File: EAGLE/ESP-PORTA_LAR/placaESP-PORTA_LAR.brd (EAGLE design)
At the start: 53.3 x 42.9 mm, 18 parts

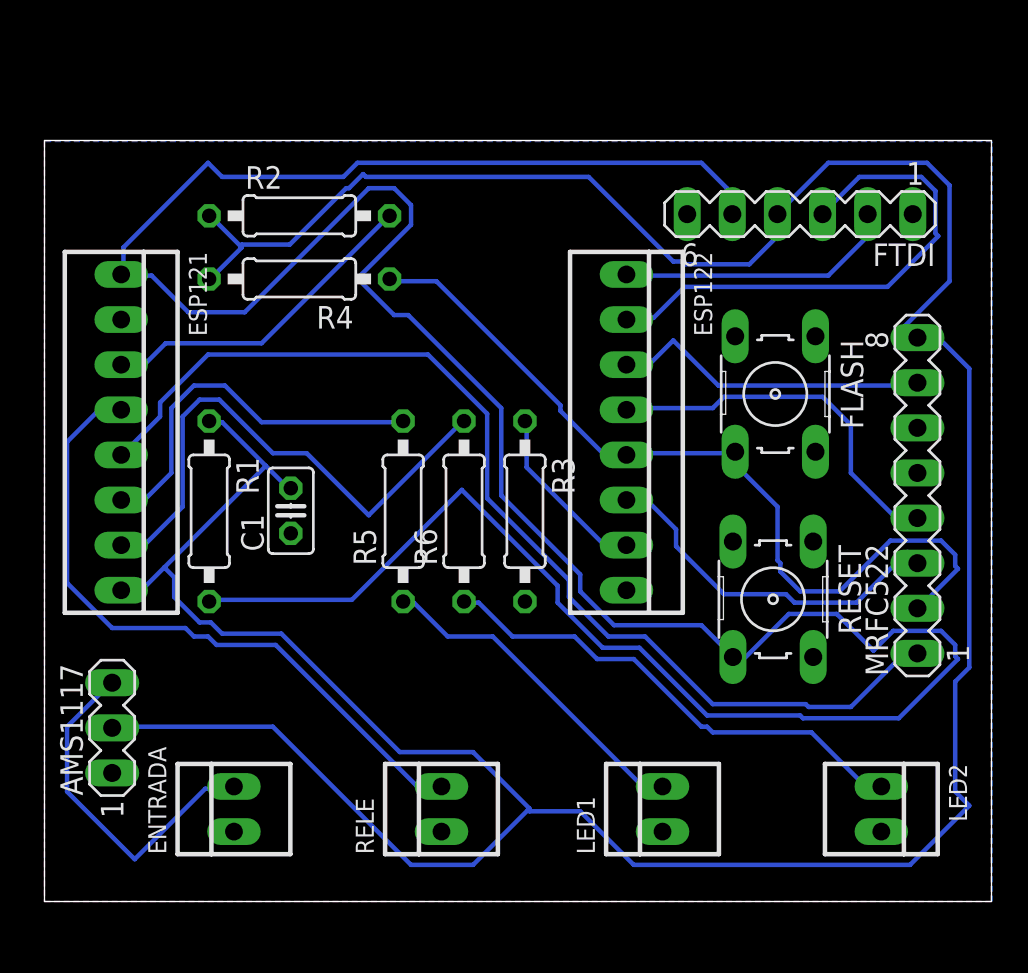
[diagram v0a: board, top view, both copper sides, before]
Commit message: Nova Placa
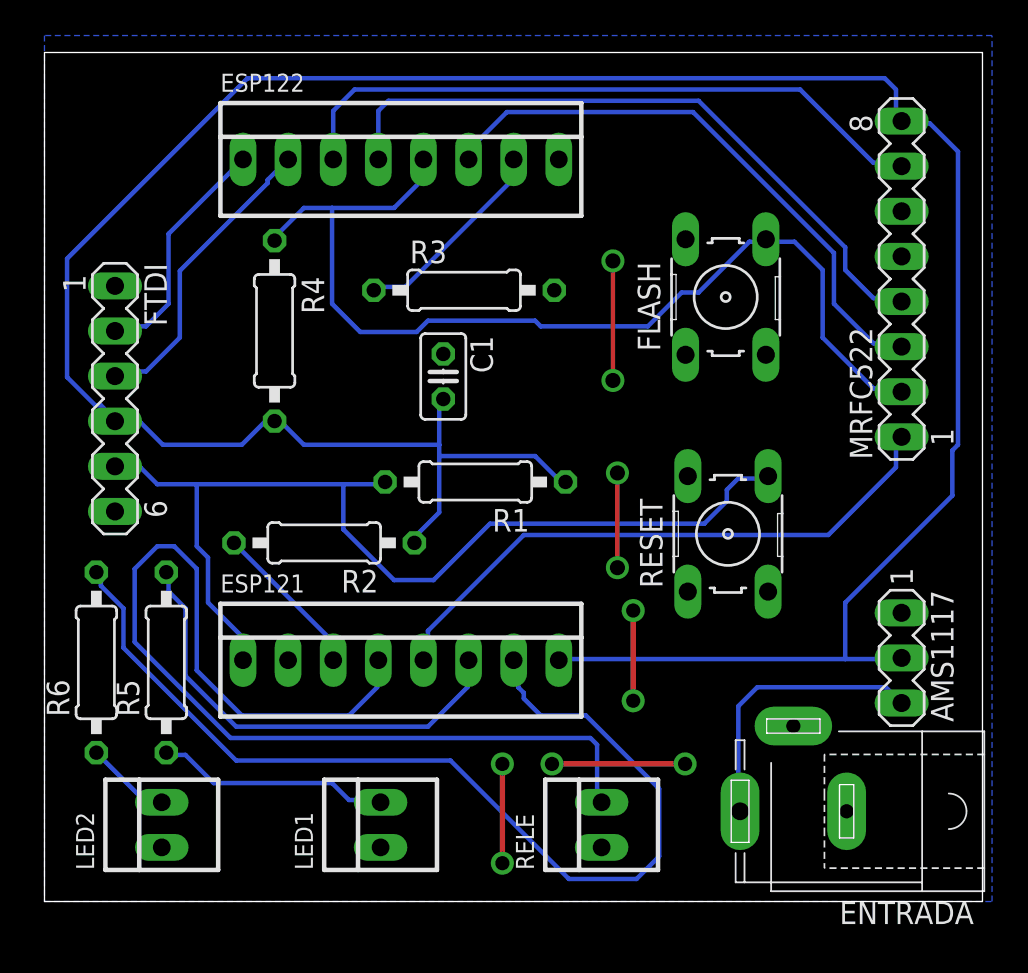
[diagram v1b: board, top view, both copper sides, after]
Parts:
- ENTRADA: value 1 -> (none); device con-molex:22-23-2021 -> con-jack:SPC4077
- moved AMS1117 44.6 mm to (48.3, 13.7), turned to 270 degrees
- moved LED2 40.5 mm to (6.60, 4.32), turned to 90 degrees
- moved FTDI 39.9 mm to (3.97, 28.3), turned to 270 degrees
- moved ENTRADA 31.5 mm to (42.2, 5.08), turned to 180 degrees
- moved R6 22.4 mm to (2.92, 13.5)
- moved ESP121 20.3 mm to (20.1, 13.6), turned to 0 degrees
- moved ESP122 19.9 mm to (20.1, 41.8), turned to 0 degrees
- moved R2 18.5 mm to (15.7, 20.2), turned to 180 degrees
- moved LED1 15.9 mm to (18.9, 4.32)
- moved R5 15.8 mm to (6.86, 13.5)
- moved R1 15.1 mm to (24.3, 23.6), turned to 180 degrees
- moved R3 12.9 mm to (23.6, 34.4), turned to 0 degrees
- moved MRFC522 12.2 mm to (48.3, 35.1)
- moved C1 11.4 mm to (22.5, 29.6), turned to 270 degrees
- moved RELE 9.06 mm to (31.4, 4.32)
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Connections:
- removed net N$6: LED2.1, R6.1
- new net N$2: LED2.2, R6.1
- net GND: now also ENTRADA.2, LED2.1; no longer LED2.2
- net IN+: now also ENTRADA.3; no longer ENTRADA.2
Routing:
- net CTS: track 168.0 -> 57.1 mm
- net VCC: track 191.6 -> 154.7 mm
- net GND: track 0.00 -> 30.2 mm, vias 0 -> 10
- net N$6: track 27.8 -> 0.00 mm
- net SDA: track 60.7 -> 33.9 mm
- net LED2: track 31.1 -> 56.9 mm
- net RELE: track 37.6 -> 59.6 mm
- net RST: track 18.1 -> 37.1 mm
- net MISO: track 21.1 -> 38.0 mm
- net TXO: track 29.7 -> 17.1 mm
- net MOSI: track 20.9 -> 33.0 mm
- net N$3: track 19.1 -> 8.92 mm
- net SCK: track 48.3 -> 57.5 mm
- net N$5: track 18.9 -> 13.2 mm
- net N$2: track 0.00 -> 4.84 mm
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- removed copper zone on layer 1, net GND
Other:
- board size 53.3 x 42.9 mm -> 52.8 x 47.8 mm
